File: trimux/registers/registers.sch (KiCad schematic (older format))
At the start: 40 parts, among them P1 CONN_02X05, U1 trimux, U2 trimux, U3 trimux, U4 trimux, U5 trimux, U6 trimux, U7 LM324

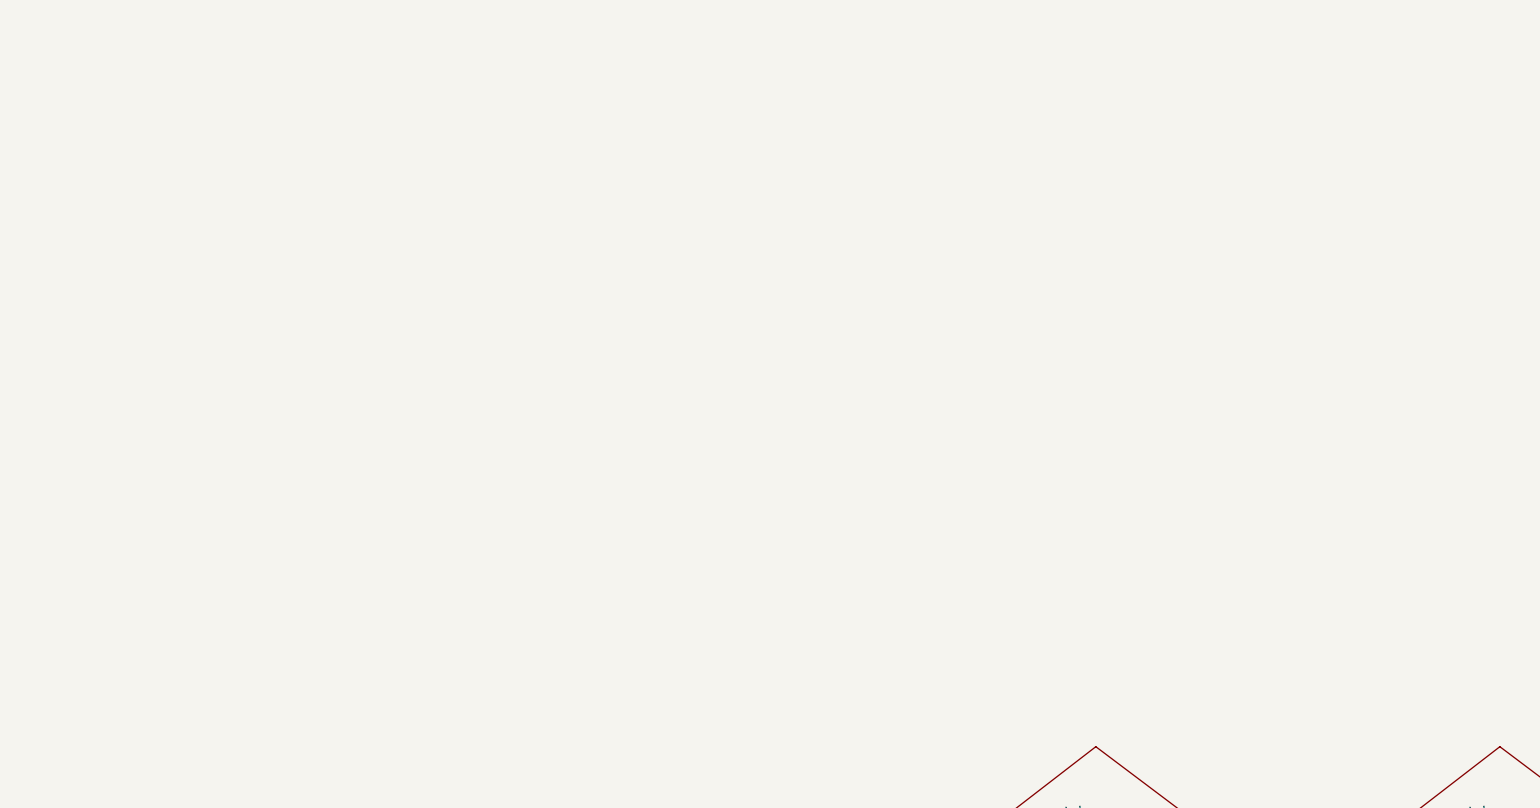
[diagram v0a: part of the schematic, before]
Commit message: adapter board final routing
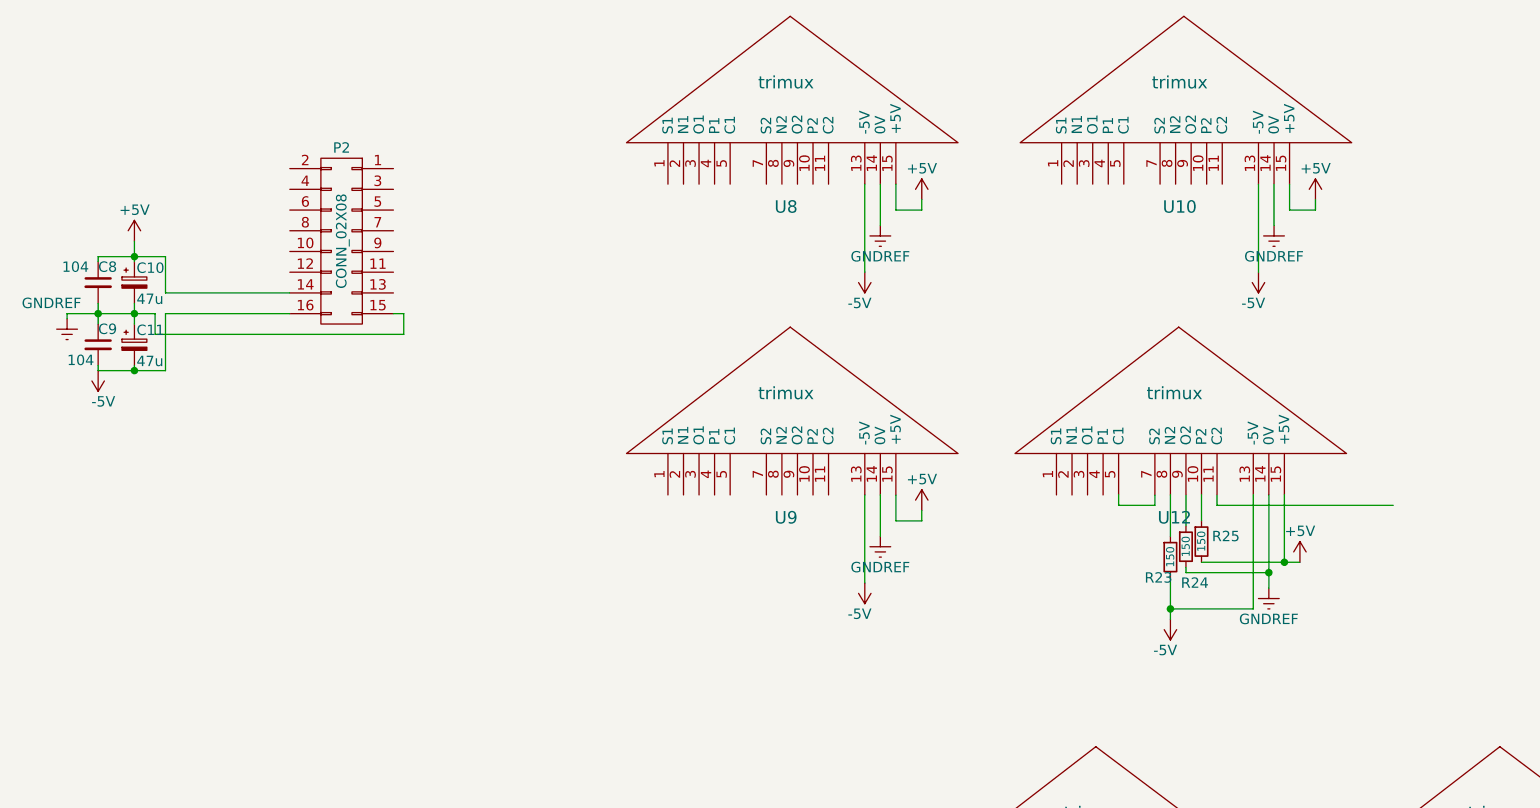
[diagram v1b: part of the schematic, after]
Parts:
- added C10, C11: 47u, Capacitors_THT:CP_Radial_D5.0mm_P2.50mm, symbol CP_Small
- added C8, C9: 104, Capacitors_SMD:C_1206_HandSoldering, symbol C_Small
- added P2: CONN_02X08, symbol CONN_02X08
- added R23, R24, R25: 150, Resistors_SMD:R_1206_HandSoldering, symbol R_Small
- added U10, U12, U8, U9: trimux, trimux:trimux1x15_2.54, symbol trimux
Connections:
- net +5V: now also C10.1, C8.1, P2.14 (P14), R25.2, U10.15 (+5V), U12.15 (+5V), U8.15 (+5V), U9.15 (+5V)
- net -5V: now also C11.2, C9.2, P2.16 (P16), R23.2, U10.13 (-5V), U12.13 (-5V), U8.13 (-5V), U9.13 (-5V)
- net GNDREF: now also C10.2, C11.1, C8.2, C9.1, P2.15 (P15), R24.2, U10.14 (0V), U12.14 (0V), U8.14 (0V), U9.14 (0V)
- new net: R25.1, U12.10 (P2)
- new net: U12.5 (C1), U12.7 (S2)
- new net: R23.1, U12.8 (N2)
- new net: R24.1, U12.9 (O2)

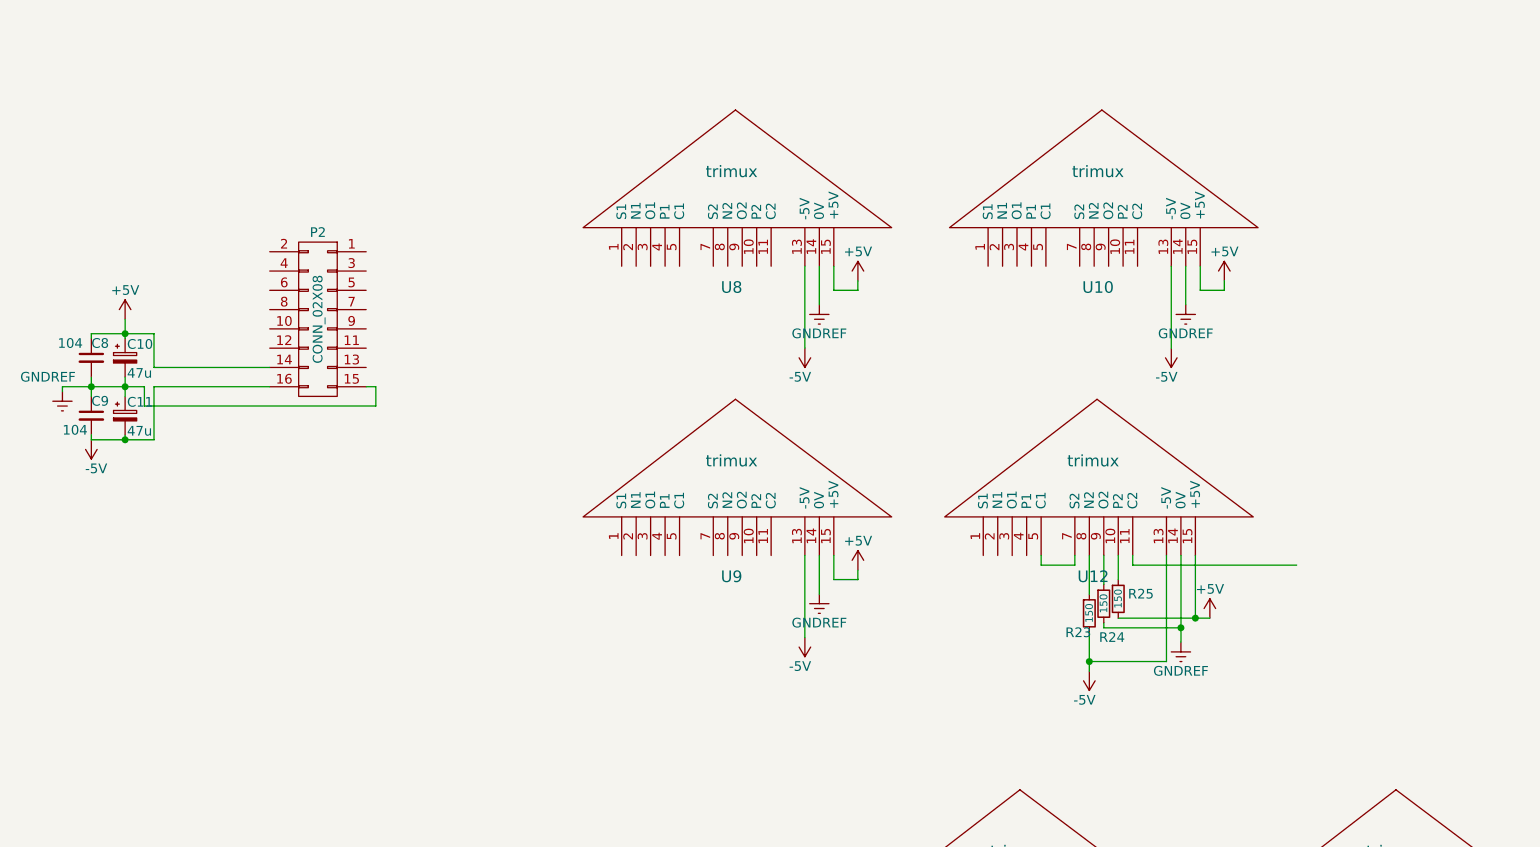
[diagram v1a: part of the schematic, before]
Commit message: memory
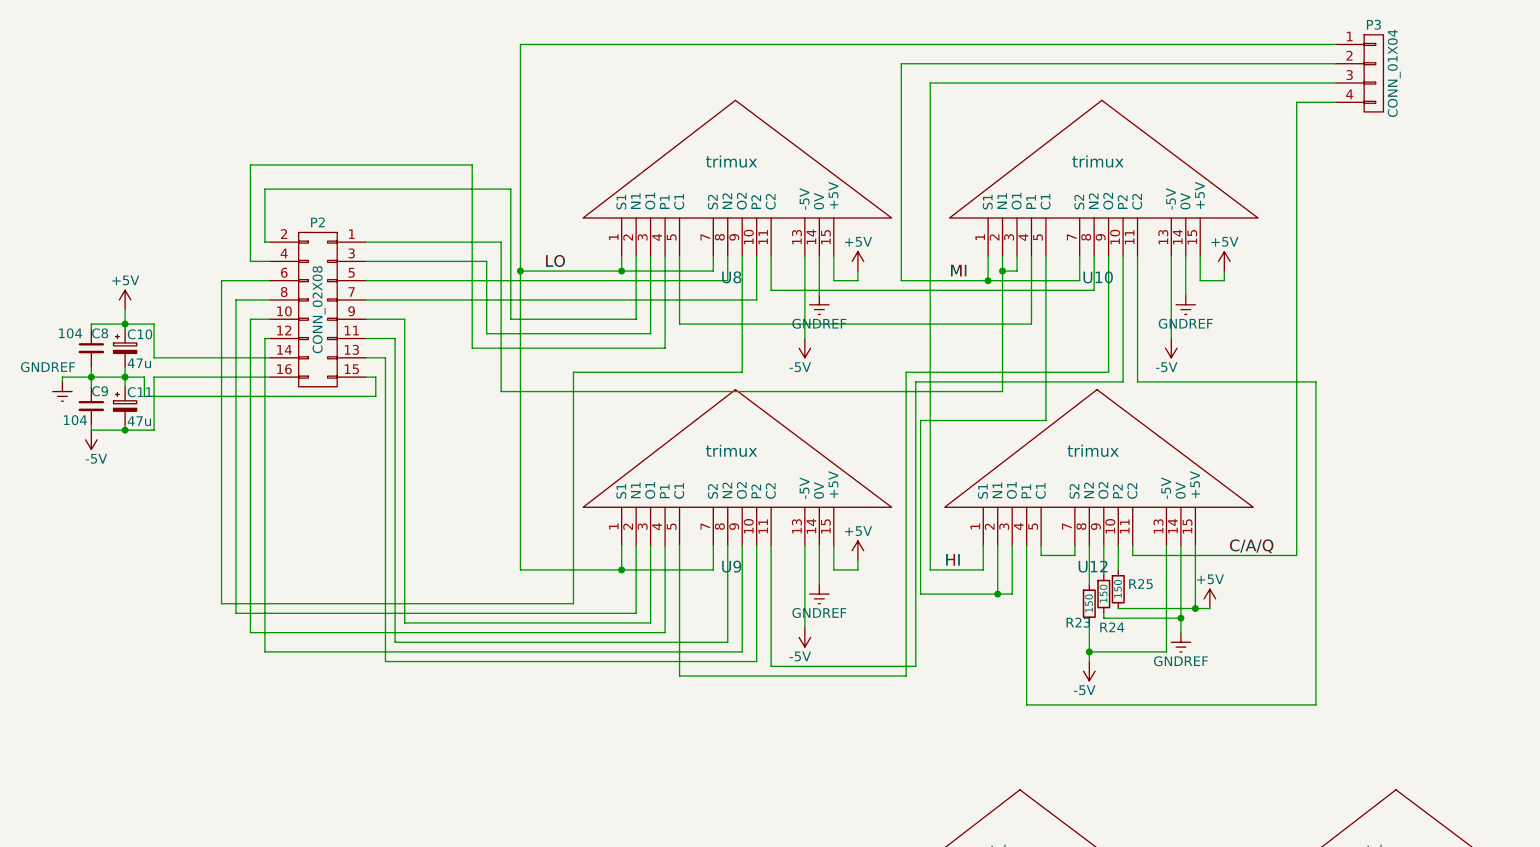
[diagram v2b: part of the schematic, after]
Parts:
- added P3: CONN_01X04, Pin_Headers:Pin_Header_Straight_1x04_Pitch2.54mm, symbol CONN_01X04
- C1, C10, C11, C2: footprint Capacitors_THT:CP_Radial_D5.0mm_P2.50mm -> Capacitors_THT:CP_Radial_D5.0mm_P2.00mm
- P2: footprint (none) -> registers:IDC16
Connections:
- net at P2.1 (P1): now also U10.2 (N1), U10.3 (O1)
- net at P2.10 (P10): now also U9.4 (P1)
- net at P2.11 (P11): now also U9.8 (N2)
- net at P2.12 (P12): now also U9.9 (O2)
- net at P2.13 (P13): now also U9.10 (P2)
- net at P2.2 (P2): now also U8.2 (N1)
- net at P2.3 (P3): now also U8.3 (O1)
- net at P2.4 (P4): now also U8.4 (P1)
- net at P2.5 (P5): now also U8.8 (N2)
- net at P2.6 (P6): now also U8.9 (O2)
- net at P2.7 (P7): now also U8.10 (P2)
- net at P2.8 (P8): now also U9.2 (N1)
- net at P2.9 (P9): now also U9.3 (O1)
- net HI: now reaches U12.1 (S1)
- net HI: now also P3.3 (P3)
- net C/A/Q: now reaches U12.11 (C2)
- net C/A/Q: now also P3.4 (P4)
- net at U12.2 (N1): now also U10.5 (C1), U12.3 (O1)
- net at U12.4 (P1): now also U10.11 (C2)
- net MI: now reaches U10.1 (S1)
- net MI: now also U10.7 (S2), P3.2 (P2)
- net at U10.10 (P2): now also U9.11 (C2)
- net at U10.4 (P1): now also U8.5 (C1)
- net at U10.8 (N2): now also U8.11 (C2)
- net at U10.9 (O2): now also U9.5 (C1)
- net LO: now reaches U8.1 (S1)
- net LO: now also U8.7 (S2), U9.1 (S1), U9.7 (S2), P3.1 (P1)
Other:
- moved on the sheet: C10, C11, C8, C9, P2, R23, R24, R25, U10, U12, U8, U9
